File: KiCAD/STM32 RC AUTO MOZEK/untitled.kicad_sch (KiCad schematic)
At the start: 7 parts, among them J10 Conn_01x05_Socket, U12 STM32F411RCTx, U6 NRF24L01_Breakout

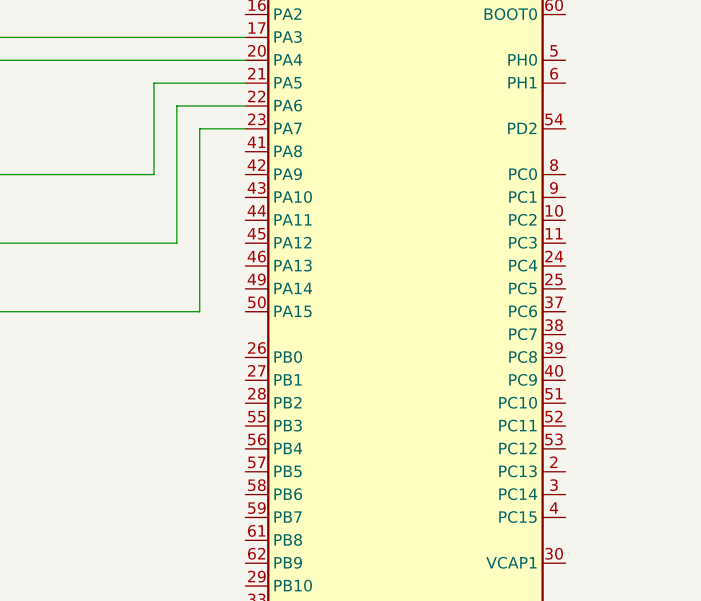
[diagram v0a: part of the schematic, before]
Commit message: Multi ADD
Completed work version of code and did more work on schematic
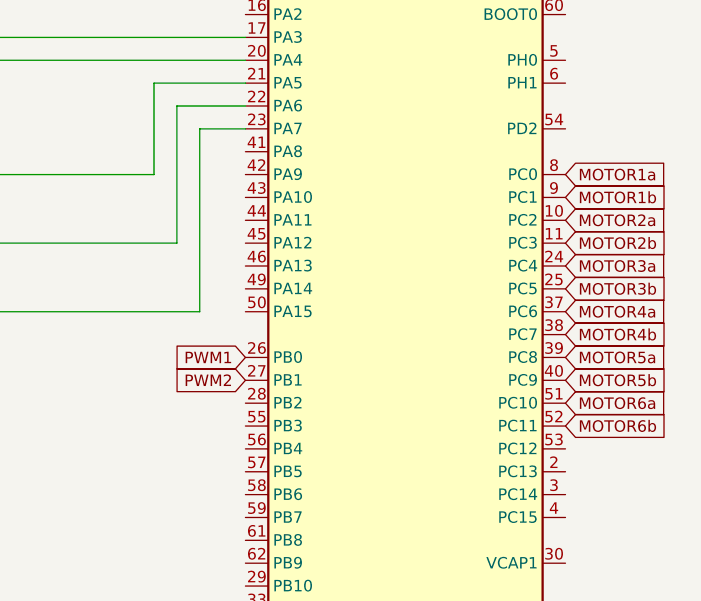
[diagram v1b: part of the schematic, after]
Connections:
- net MOTOR2a: now reaches U12.10 (PC2)
- net MOTOR2b: now reaches U12.11 (PC3)
- net MOTOR3a: now reaches U12.24 (PC4)
- net MOTOR3b: now reaches U12.25 (PC5)
- net PWM1: now reaches U12.26 (PB0)
- net PWM2: now reaches U12.27 (PB1)
- net MOTOR4a: now reaches U12.37 (PC6)
- net MOTOR4b: now reaches U12.38 (PC7)
- net MOTOR5a: now reaches U12.39 (PC8)
- net MOTOR5b: now reaches U12.40 (PC9)
- net MOTOR6a: now reaches U12.51 (PC10)
- net MOTOR6b: now reaches U12.52 (PC11)
- net MOTOR1a: now reaches U12.8 (PC0)
- net MOTOR1b: now reaches U12.9 (PC1)

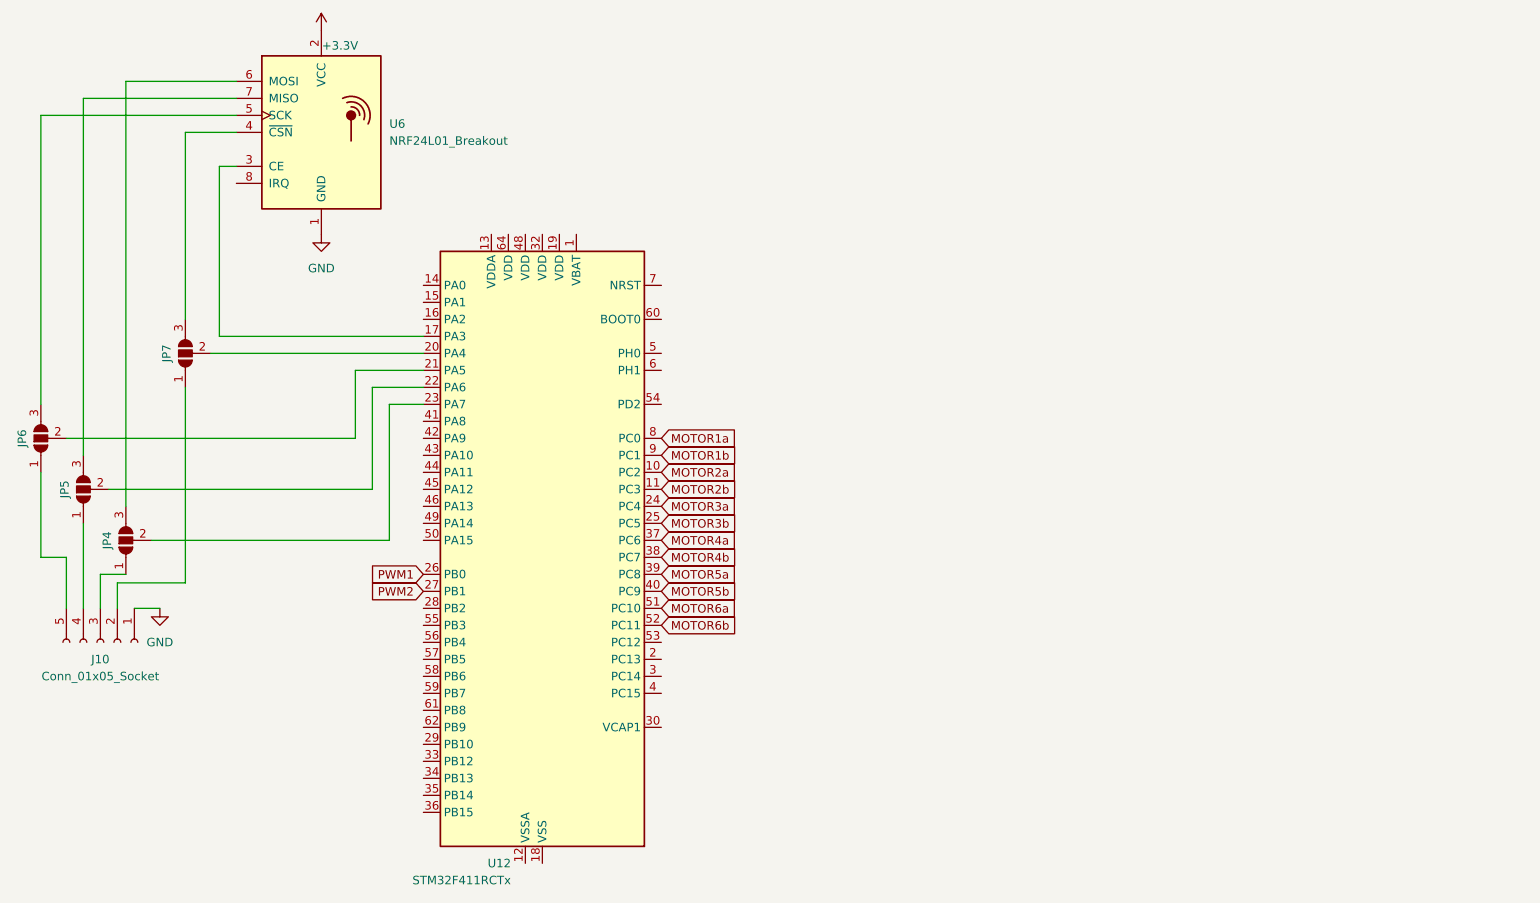
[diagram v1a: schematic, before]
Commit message: .
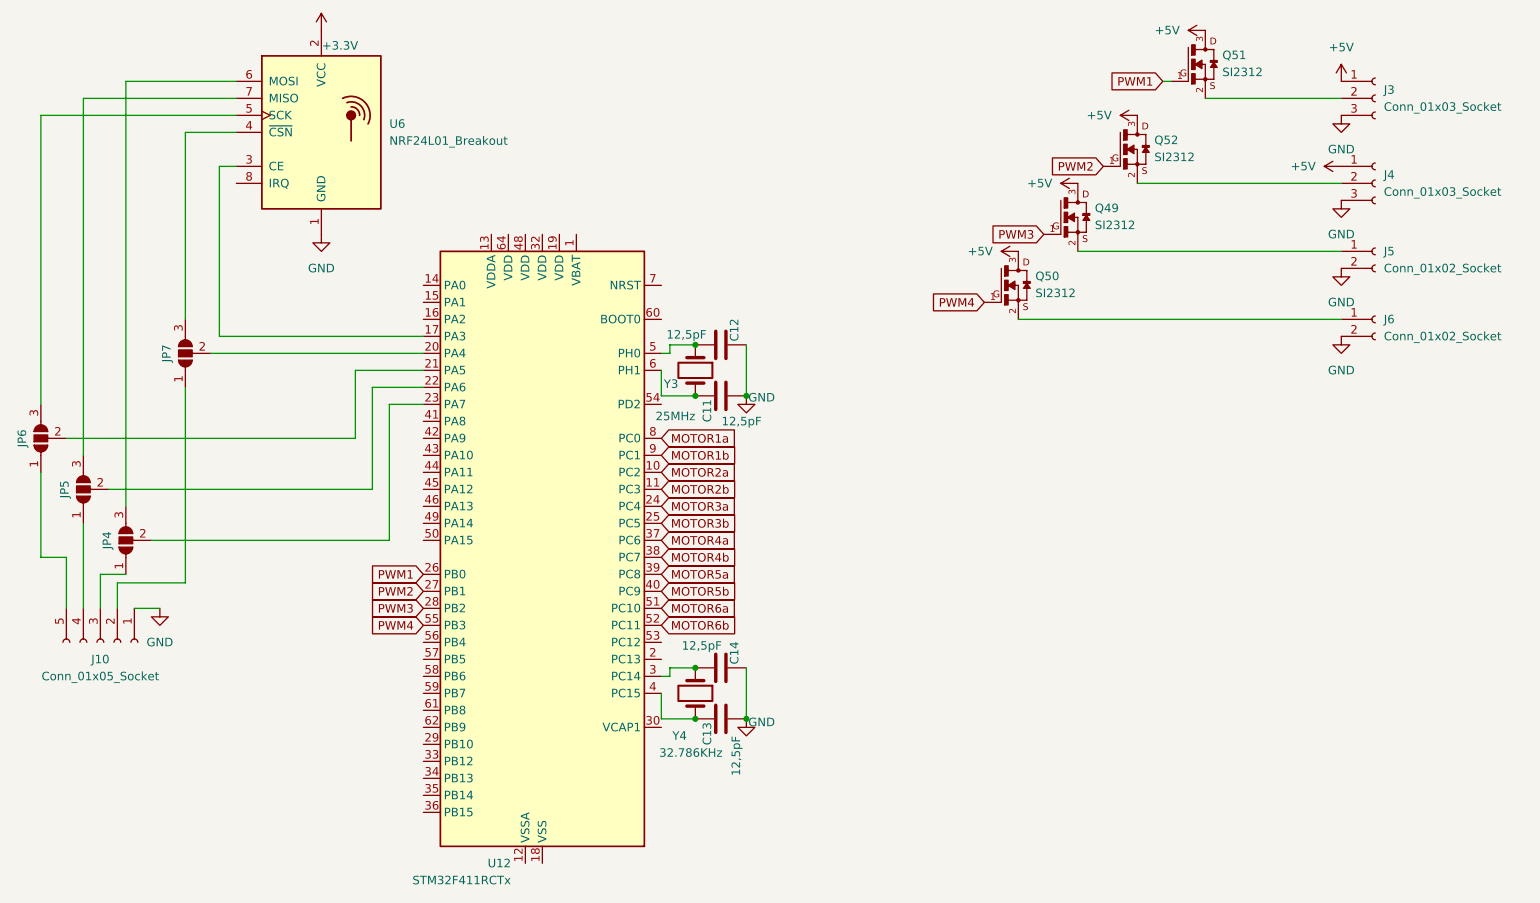
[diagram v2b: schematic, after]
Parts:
- added C11, C12, C13, C14: 12,5pF, Capacitor_SMD:C_0805_2012Metric_Pad1.18x1.45mm_HandSolder, symbol Device:C
- added J3, J4: Conn_01x03_Socket, Connector_JST:JST_XH_B3B-XH-A_1x03_P2.50mm_Vertical, symbol Connector:Conn_01x03_Socket
- added J5, J6: Conn_01x02_Socket, Connector_JST:JST_XH_B2B-XH-A_1x02_P2.50mm_Vertical, symbol Connector:Conn_01x02_Socket
- added Q49, Q50, Q51, Q52: SI2312, SI2312:SOT23, symbol SI2312:SI2312
- added Y3: 25MHz, Crystal:Crystal_SMD_HC49-SD, symbol Device:Crystal
- added Y4: 32.786KHz, Crystal:Crystal_DS26_D2.0mm_L6.0mm_Horizontal, symbol Device:Crystal
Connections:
- net GND: now also C11.2, C12.1, C13.2, C14.1, J3.3 (Pin_3), J4.3 (Pin_3), J5.2 (Pin_2), J6.2 (Pin_2)
- net PWM1: now also Q51.1
- net PWM2: now also Q52.1
- net PWM3: now reaches U12.28 (PB2)
- net PWM3: now also Q49.1
- net at U12.3 (PC14): now also C14.2, Y4.1
- net at U12.4 (PC15): now also C13.1, Y4.2
- net at U12.5 (PH0): now also C12.2, Y3.1
- net PWM4: now reaches U12.55 (PB3)
- net PWM4: now also Q50.1
- net at U12.6 (PH1): now also C11.1, Y3.2
- new net: J5.1 (Pin_1), Q49.2
- new net: J3.2 (Pin_2), Q51.2
- new net: J6.1 (Pin_1), Q50.2
- new net: J4.2 (Pin_2), Q52.2
- new net +5V: J3.1 (Pin_1), J4.1 (Pin_1), Q49.3, Q50.3, Q51.3, Q52.3
